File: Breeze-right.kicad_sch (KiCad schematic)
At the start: 103 parts, among them J1 J, SW1 CHOCXHSPCB-1U, SW10 CHOCXHSPCB-1U, SW11 CHOCXHSPCB-1U, SW12 CHOCXHSPCB-1U, SW13 CHOCXHSPCB-1U, SW14 CHOCXHSPCB-1U, SW15 CHOCXHSPCB-1U, SW16 CHOCXHSPCB-1U, SW17 CHOCXHSPCB-1U, SW18 CHOCXHSPCB-1U, SW19 CHOCXHSPCB-1U, SW2 CHOCXHSPCB-1U, SW20 CHOCXHSPCB-1U, SW21 CHOCXHSPCB-1U, SW22 CHOCXHSPCB-1U, SW23 CHOCXHSPCB-1U, SW24 CHOCXHSPCB-1U, SW3 CHOCXHSPCB-1U, SW4 CHOCXHSPCB-1U, SW5 CHOCXHSPCB-1U, SW6 CHOCXHSPCB-1U, SW7 CHOCXHSPCB-1U, SW8 CHOCXHSPCB-1U, SW9 CHOCXHSPCB-1U, U1 NRF Supermini

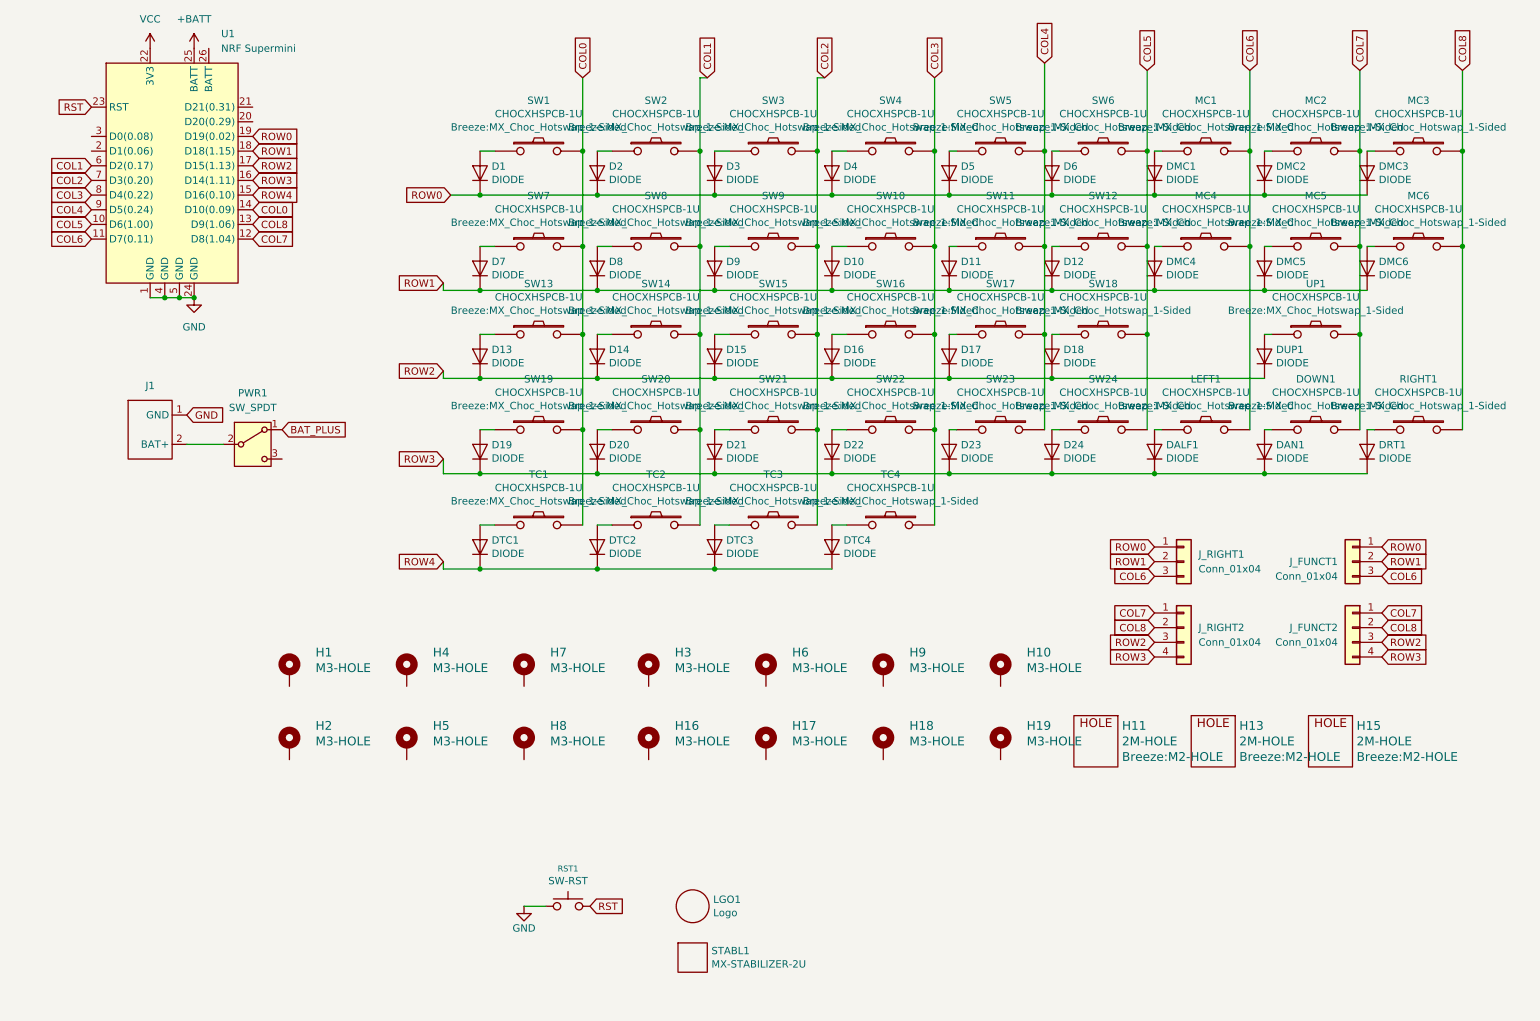
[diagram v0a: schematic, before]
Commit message: done
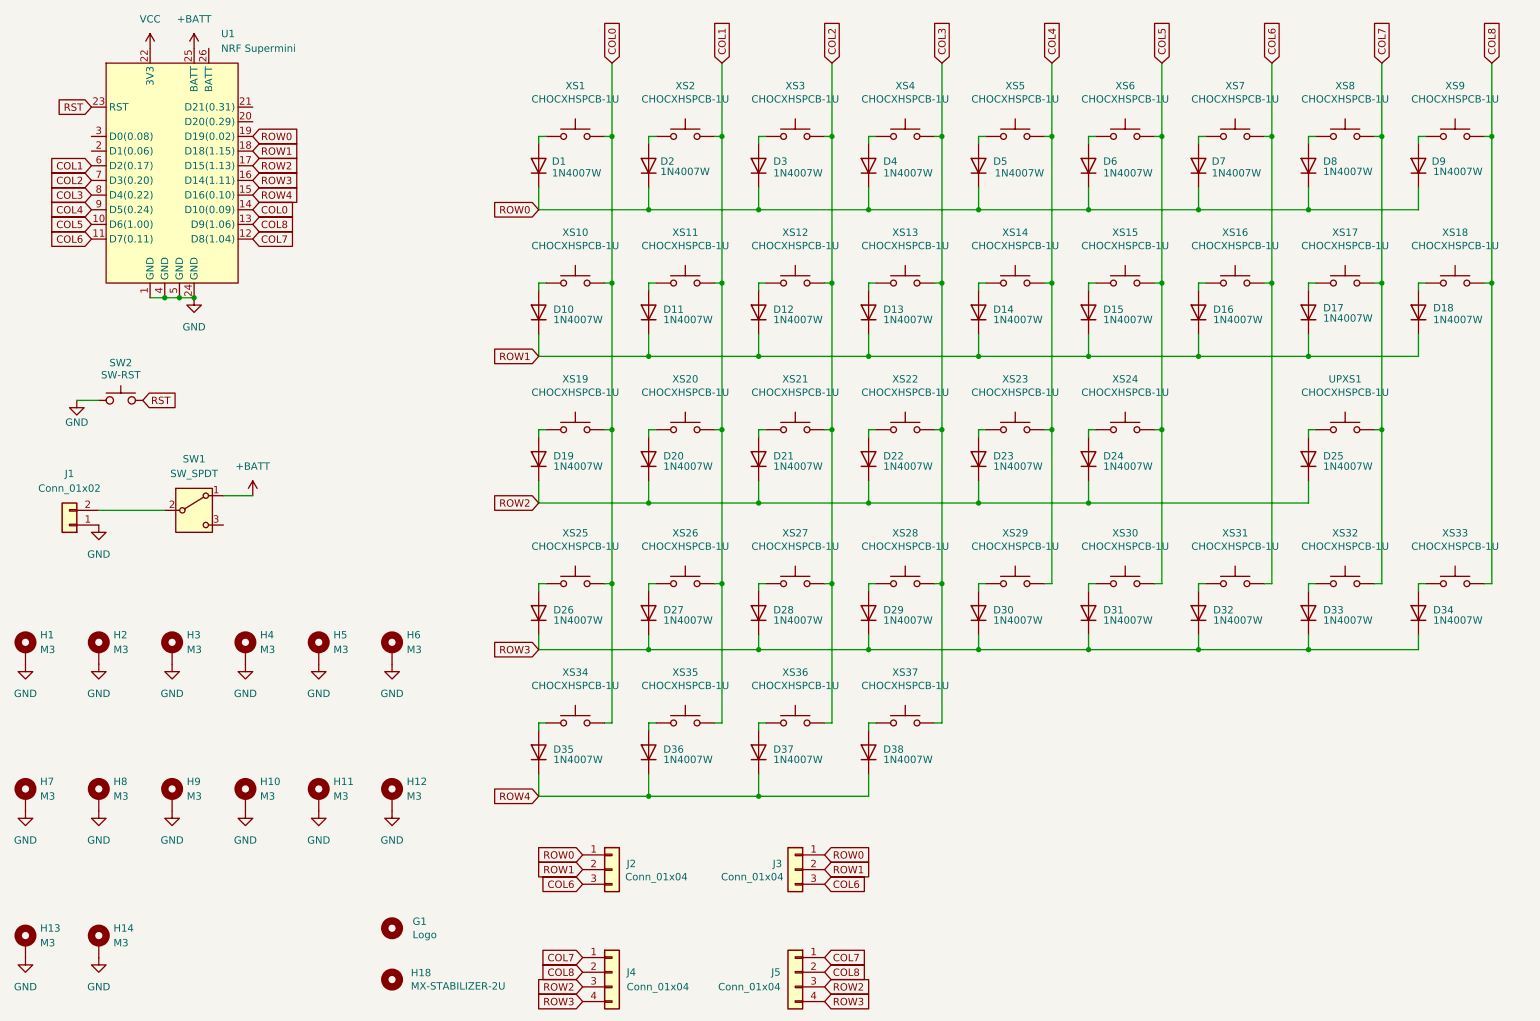
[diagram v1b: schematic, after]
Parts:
- removed H11, H13, H15: 2M-HOLE, Breeze:M2-HOLE, symbol Breeze-rescue:2M-HOLE-Breeze-rescue
- removed H16, H17, H18, H19: M3-HOLE, Breeze:M3-HOLE, symbol Mechanical:MountingHole_Pad
- removed J1: J, Breeze:BATT_PADS, symbol Breeze:BATT_PADS
- removed PWR1: SW_SPDT, Breeze:SS12D00, symbol Switch:SW_SPDT
- added H11, H12, H13, H14: M3, MountingHole:MountingHole_3.2mm_M3_ISO7380_Pad, symbol Mechanical:MountingHole_Pad
- added J1: Conn_01x02, Breeze:BATT_PADS, symbol Connector_Generic:Conn_01x02
- added SW1: SW_SPDT, Breeze:SS12D00, symbol Switch:SW_SPDT
- D1, D2, D3, D4, D5, D6: value DIODE -> 1N4007W; footprint Breeze:SOD-123FL -> Breeze:SOD-123FL_L2.7-W1.8-LS3.7-RD; symbol Breeze-rescue:Diode-cache-Merkaba_Rev0-rescue-Breeze-rescue -> Diode:1N4007
- D10: renamed from D7; value DIODE -> 1N4007W; footprint Breeze:SOD-123FL -> Breeze:SOD-123FL_L2.7-W1.8-LS3.7-RD; symbol Breeze-rescue:Diode-cache-Merkaba_Rev0-rescue-Breeze-rescue -> Diode:1N4007
- D11: renamed from D8; value DIODE -> 1N4007W; footprint Breeze:SOD-123FL -> Breeze:SOD-123FL_L2.7-W1.8-LS3.7-RD; symbol Breeze-rescue:Diode-cache-Merkaba_Rev0-rescue-Breeze-rescue -> Diode:1N4007
- D12: renamed from D9; value DIODE -> 1N4007W; footprint Breeze:SOD-123FL -> Breeze:SOD-123FL_L2.7-W1.8-LS3.7-RD; symbol Breeze-rescue:Diode-cache-Merkaba_Rev0-rescue-Breeze-rescue -> Diode:1N4007
- D13: renamed from D10; value DIODE -> 1N4007W; footprint Breeze:SOD-123FL -> Breeze:SOD-123FL_L2.7-W1.8-LS3.7-RD; symbol Breeze-rescue:Diode-cache-Merkaba_Rev0-rescue-Breeze-rescue -> Diode:1N4007
- D14: renamed from D11; value DIODE -> 1N4007W; footprint Breeze:SOD-123FL -> Breeze:SOD-123FL_L2.7-W1.8-LS3.7-RD; symbol Breeze-rescue:Diode-cache-Merkaba_Rev0-rescue-Breeze-rescue -> Diode:1N4007
- D15: renamed from D12; value DIODE -> 1N4007W; footprint Breeze:SOD-123FL -> Breeze:SOD-123FL_L2.7-W1.8-LS3.7-RD; symbol Breeze-rescue:Diode-cache-Merkaba_Rev0-rescue-Breeze-rescue -> Diode:1N4007
- D16: renamed from DMC4; value DIODE -> 1N4007W; footprint Breeze:SOD-123FL -> Breeze:SOD-123FL_L2.7-W1.8-LS3.7-RD; symbol Breeze-rescue:Diode-cache-Merkaba_Rev0-rescue-Breeze-rescue -> Diode:1N4007
- D17: renamed from DMC5; value DIODE -> 1N4007W; footprint Breeze:SOD-123FL -> Breeze:SOD-123FL_L2.7-W1.8-LS3.7-RD; symbol Breeze-rescue:Diode-cache-Merkaba_Rev0-rescue-Breeze-rescue -> Diode:1N4007
- D18: renamed from DMC6; value DIODE -> 1N4007W; footprint Breeze:SOD-123FL -> Breeze:SOD-123FL_L2.7-W1.8-LS3.7-RD; symbol Breeze-rescue:Diode-cache-Merkaba_Rev0-rescue-Breeze-rescue -> Diode:1N4007
- D19: renamed from D13; value DIODE -> 1N4007W; footprint Breeze:SOD-123FL -> Breeze:SOD-123FL_L2.7-W1.8-LS3.7-RD; symbol Breeze-rescue:Diode-cache-Merkaba_Rev0-rescue-Breeze-rescue -> Diode:1N4007
- D20: renamed from D14; value DIODE -> 1N4007W; footprint Breeze:SOD-123FL -> Breeze:SOD-123FL_L2.7-W1.8-LS3.7-RD; symbol Breeze-rescue:Diode-cache-Merkaba_Rev0-rescue-Breeze-rescue -> Diode:1N4007
- D21: renamed from D15; value DIODE -> 1N4007W; footprint Breeze:SOD-123FL -> Breeze:SOD-123FL_L2.7-W1.8-LS3.7-RD; symbol Breeze-rescue:Diode-cache-Merkaba_Rev0-rescue-Breeze-rescue -> Diode:1N4007
- D22: renamed from D16; value DIODE -> 1N4007W; footprint Breeze:SOD-123FL -> Breeze:SOD-123FL_L2.7-W1.8-LS3.7-RD; symbol Breeze-rescue:Diode-cache-Merkaba_Rev0-rescue-Breeze-rescue -> Diode:1N4007
- D23: renamed from D17; value DIODE -> 1N4007W; footprint Breeze:SOD-123FL -> Breeze:SOD-123FL_L2.7-W1.8-LS3.7-RD; symbol Breeze-rescue:Diode-cache-Merkaba_Rev0-rescue-Breeze-rescue -> Diode:1N4007
- D24: renamed from D18; value DIODE -> 1N4007W; footprint Breeze:SOD-123FL -> Breeze:SOD-123FL_L2.7-W1.8-LS3.7-RD; symbol Breeze-rescue:Diode-cache-Merkaba_Rev0-rescue-Breeze-rescue -> Diode:1N4007
- D25: renamed from DUP1; value DIODE -> 1N4007W; footprint Breeze:SOD-123FL -> Breeze:SOD-123FL_L2.7-W1.8-LS3.7-RD; symbol Breeze-rescue:Diode-cache-Merkaba_Rev0-rescue-Breeze-rescue -> Diode:1N4007
- D26: renamed from D19; value DIODE -> 1N4007W; footprint Breeze:SOD-123FL -> Breeze:SOD-123FL_L2.7-W1.8-LS3.7-RD; symbol Breeze-rescue:Diode-cache-Merkaba_Rev0-rescue-Breeze-rescue -> Diode:1N4007
- D27: renamed from D20; value DIODE -> 1N4007W; footprint Breeze:SOD-123FL -> Breeze:SOD-123FL_L2.7-W1.8-LS3.7-RD; symbol Breeze-rescue:Diode-cache-Merkaba_Rev0-rescue-Breeze-rescue -> Diode:1N4007
- D28: renamed from D21; value DIODE -> 1N4007W; footprint Breeze:SOD-123FL -> Breeze:SOD-123FL_L2.7-W1.8-LS3.7-RD; symbol Breeze-rescue:Diode-cache-Merkaba_Rev0-rescue-Breeze-rescue -> Diode:1N4007
- D29: renamed from D22; value DIODE -> 1N4007W; footprint Breeze:SOD-123FL -> Breeze:SOD-123FL_L2.7-W1.8-LS3.7-RD; symbol Breeze-rescue:Diode-cache-Merkaba_Rev0-rescue-Breeze-rescue -> Diode:1N4007
- D30: renamed from D23; value DIODE -> 1N4007W; footprint Breeze:SOD-123FL -> Breeze:SOD-123FL_L2.7-W1.8-LS3.7-RD; symbol Breeze-rescue:Diode-cache-Merkaba_Rev0-rescue-Breeze-rescue -> Diode:1N4007
- D31: renamed from D24; value DIODE -> 1N4007W; footprint Breeze:SOD-123FL -> Breeze:SOD-123FL_L2.7-W1.8-LS3.7-RD; symbol Breeze-rescue:Diode-cache-Merkaba_Rev0-rescue-Breeze-rescue -> Diode:1N4007
- D32: renamed from DALF1; value DIODE -> 1N4007W; footprint Breeze:SOD-123FL -> Breeze:SOD-123FL_L2.7-W1.8-LS3.7-RD; symbol Breeze-rescue:Diode-cache-Merkaba_Rev0-rescue-Breeze-rescue -> Diode:1N4007
- D33: renamed from DAN1; value DIODE -> 1N4007W; footprint Breeze:SOD-123FL -> Breeze:SOD-123FL_L2.7-W1.8-LS3.7-RD; symbol Breeze-rescue:Diode-cache-Merkaba_Rev0-rescue-Breeze-rescue -> Diode:1N4007
- D34: renamed from DRT1; value DIODE -> 1N4007W; footprint Breeze:SOD-123FL -> Breeze:SOD-123FL_L2.7-W1.8-LS3.7-RD; symbol Breeze-rescue:Diode-cache-Merkaba_Rev0-rescue-Breeze-rescue -> Diode:1N4007
- D35: renamed from DTC1; value DIODE -> 1N4007W; footprint Breeze:SOD-123FL -> Breeze:SOD-123FL_L2.7-W1.8-LS3.7-RD; symbol Breeze-rescue:Diode-cache-Merkaba_Rev0-rescue-Breeze-rescue -> Diode:1N4007
- D36: renamed from DTC2; value DIODE -> 1N4007W; footprint Breeze:SOD-123FL -> Breeze:SOD-123FL_L2.7-W1.8-LS3.7-RD; symbol Breeze-rescue:Diode-cache-Merkaba_Rev0-rescue-Breeze-rescue -> Diode:1N4007
- D37: renamed from DTC3; value DIODE -> 1N4007W; footprint Breeze:SOD-123FL -> Breeze:SOD-123FL_L2.7-W1.8-LS3.7-RD; symbol Breeze-rescue:Diode-cache-Merkaba_Rev0-rescue-Breeze-rescue -> Diode:1N4007
- D38: renamed from DTC4; value DIODE -> 1N4007W; footprint Breeze:SOD-123FL -> Breeze:SOD-123FL_L2.7-W1.8-LS3.7-RD; symbol Breeze-rescue:Diode-cache-Merkaba_Rev0-rescue-Breeze-rescue -> Diode:1N4007
- D7: renamed from DMC1; value DIODE -> 1N4007W; footprint Breeze:SOD-123FL -> Breeze:SOD-123FL_L2.7-W1.8-LS3.7-RD; symbol Breeze-rescue:Diode-cache-Merkaba_Rev0-rescue-Breeze-rescue -> Diode:1N4007
- D8: renamed from DMC2; value DIODE -> 1N4007W; footprint Breeze:SOD-123FL -> Breeze:SOD-123FL_L2.7-W1.8-LS3.7-RD; symbol Breeze-rescue:Diode-cache-Merkaba_Rev0-rescue-Breeze-rescue -> Diode:1N4007
- D9: renamed from DMC3; value DIODE -> 1N4007W; footprint Breeze:SOD-123FL -> Breeze:SOD-123FL_L2.7-W1.8-LS3.7-RD; symbol Breeze-rescue:Diode-cache-Merkaba_Rev0-rescue-Breeze-rescue -> Diode:1N4007
- G1: renamed from LGO1; symbol Breeze-rescue:Logo-Breeze-rescue -> Mechanical:MountingHole; now left out of the parts list
- H1, H10, H3, H4, H6, H7, H9: value M3-HOLE -> M3; footprint Breeze:M3-HOLE -> MountingHole:MountingHole_3.2mm_M3_ISO7380_Pad
- H18: renamed from STABL1; symbol Breeze-rescue:MX-STABILIZER-2U-Merkaba_Rev0-rescue-Breeze-rescue -> Mechanical:MountingHole; now left out of the parts list
- H2, H5, H8: value M3-HOLE -> M3; footprint Breeze:M3-HOLE -> MountingHole:MountingHole_3.2mm_M3_ISO7380_Pad_TopOnly
- UPXS1: renamed from UP1; symbol Breeze-rescue:CHOCXHSPCB-1U-cache-Merkaba_Rev0-rescue-Breeze-rescue -> Switch:SW_Push
- XS1: renamed from SW1; symbol Breeze-rescue:CHOCXHSPCB-1U-cache-Merkaba_Rev0-rescue-Breeze-rescue -> Switch:SW_Push
- XS10: renamed from SW7; symbol Breeze-rescue:CHOCXHSPCB-1U-cache-Merkaba_Rev0-rescue-Breeze-rescue -> Switch:SW_Push
- XS11: renamed from SW8; symbol Breeze-rescue:CHOCXHSPCB-1U-cache-Merkaba_Rev0-rescue-Breeze-rescue -> Switch:SW_Push
- XS12: renamed from SW9; symbol Breeze-rescue:CHOCXHSPCB-1U-cache-Merkaba_Rev0-rescue-Breeze-rescue -> Switch:SW_Push
- XS13: renamed from SW10; symbol Breeze-rescue:CHOCXHSPCB-1U-cache-Merkaba_Rev0-rescue-Breeze-rescue -> Switch:SW_Push
- XS14: renamed from SW11; symbol Breeze-rescue:CHOCXHSPCB-1U-cache-Merkaba_Rev0-rescue-Breeze-rescue -> Switch:SW_Push
- XS15: renamed from SW12; symbol Breeze-rescue:CHOCXHSPCB-1U-cache-Merkaba_Rev0-rescue-Breeze-rescue -> Switch:SW_Push
- XS16: renamed from MC4; symbol Breeze-rescue:CHOCXHSPCB-1U-cache-Merkaba_Rev0-rescue-Breeze-rescue -> Switch:SW_Push
- XS17: renamed from MC5; symbol Breeze-rescue:CHOCXHSPCB-1U-cache-Merkaba_Rev0-rescue-Breeze-rescue -> Switch:SW_Push
- XS18: renamed from MC6; symbol Breeze-rescue:CHOCXHSPCB-1U-cache-Merkaba_Rev0-rescue-Breeze-rescue -> Switch:SW_Push
- XS19: renamed from SW13; symbol Breeze-rescue:CHOCXHSPCB-1U-cache-Merkaba_Rev0-rescue-Breeze-rescue -> Switch:SW_Push
- XS2: renamed from SW2; symbol Breeze-rescue:CHOCXHSPCB-1U-cache-Merkaba_Rev0-rescue-Breeze-rescue -> Switch:SW_Push
- XS20: renamed from SW14; symbol Breeze-rescue:CHOCXHSPCB-1U-cache-Merkaba_Rev0-rescue-Breeze-rescue -> Switch:SW_Push
- XS21: renamed from SW15; symbol Breeze-rescue:CHOCXHSPCB-1U-cache-Merkaba_Rev0-rescue-Breeze-rescue -> Switch:SW_Push
- XS22: renamed from SW16; symbol Breeze-rescue:CHOCXHSPCB-1U-cache-Merkaba_Rev0-rescue-Breeze-rescue -> Switch:SW_Push
- XS23: renamed from SW17; symbol Breeze-rescue:CHOCXHSPCB-1U-cache-Merkaba_Rev0-rescue-Breeze-rescue -> Switch:SW_Push
- XS24: renamed from SW18; symbol Breeze-rescue:CHOCXHSPCB-1U-cache-Merkaba_Rev0-rescue-Breeze-rescue -> Switch:SW_Push
- XS25: renamed from SW19; symbol Breeze-rescue:CHOCXHSPCB-1U-cache-Merkaba_Rev0-rescue-Breeze-rescue -> Switch:SW_Push
- XS26: renamed from SW20; symbol Breeze-rescue:CHOCXHSPCB-1U-cache-Merkaba_Rev0-rescue-Breeze-rescue -> Switch:SW_Push
- XS27: renamed from SW21; symbol Breeze-rescue:CHOCXHSPCB-1U-cache-Merkaba_Rev0-rescue-Breeze-rescue -> Switch:SW_Push
- XS28: renamed from SW22; symbol Breeze-rescue:CHOCXHSPCB-1U-cache-Merkaba_Rev0-rescue-Breeze-rescue -> Switch:SW_Push
- XS29: renamed from SW23; symbol Breeze-rescue:CHOCXHSPCB-1U-cache-Merkaba_Rev0-rescue-Breeze-rescue -> Switch:SW_Push
- XS3: renamed from SW3; symbol Breeze-rescue:CHOCXHSPCB-1U-cache-Merkaba_Rev0-rescue-Breeze-rescue -> Switch:SW_Push
- XS30: renamed from SW24; symbol Breeze-rescue:CHOCXHSPCB-1U-cache-Merkaba_Rev0-rescue-Breeze-rescue -> Switch:SW_Push
- XS31: renamed from LEFT1; symbol Breeze-rescue:CHOCXHSPCB-1U-cache-Merkaba_Rev0-rescue-Breeze-rescue -> Switch:SW_Push
- XS32: renamed from DOWN1; symbol Breeze-rescue:CHOCXHSPCB-1U-cache-Merkaba_Rev0-rescue-Breeze-rescue -> Switch:SW_Push
- XS33: renamed from RIGHT1; symbol Breeze-rescue:CHOCXHSPCB-1U-cache-Merkaba_Rev0-rescue-Breeze-rescue -> Switch:SW_Push
- XS34: renamed from TC1; symbol Breeze-rescue:CHOCXHSPCB-1U-cache-Merkaba_Rev0-rescue-Breeze-rescue -> Switch:SW_Push
- XS35: renamed from TC2; symbol Breeze-rescue:CHOCXHSPCB-1U-cache-Merkaba_Rev0-rescue-Breeze-rescue -> Switch:SW_Push
- XS36: renamed from TC3; symbol Breeze-rescue:CHOCXHSPCB-1U-cache-Merkaba_Rev0-rescue-Breeze-rescue -> Switch:SW_Push
- XS37: renamed from TC4; symbol Breeze-rescue:CHOCXHSPCB-1U-cache-Merkaba_Rev0-rescue-Breeze-rescue -> Switch:SW_Push
- XS4: renamed from SW4; symbol Breeze-rescue:CHOCXHSPCB-1U-cache-Merkaba_Rev0-rescue-Breeze-rescue -> Switch:SW_Push
- XS5: renamed from SW5; symbol Breeze-rescue:CHOCXHSPCB-1U-cache-Merkaba_Rev0-rescue-Breeze-rescue -> Switch:SW_Push
- XS6: renamed from SW6; symbol Breeze-rescue:CHOCXHSPCB-1U-cache-Merkaba_Rev0-rescue-Breeze-rescue -> Switch:SW_Push
- XS7: renamed from MC1; symbol Breeze-rescue:CHOCXHSPCB-1U-cache-Merkaba_Rev0-rescue-Breeze-rescue -> Switch:SW_Push
- XS8: renamed from MC2; symbol Breeze-rescue:CHOCXHSPCB-1U-cache-Merkaba_Rev0-rescue-Breeze-rescue -> Switch:SW_Push
- XS9: renamed from MC3; symbol Breeze-rescue:CHOCXHSPCB-1U-cache-Merkaba_Rev0-rescue-Breeze-rescue -> Switch:SW_Push
- renumbered J_RIGHT1 to J2, J_FUNCT1 to J3, J_RIGHT2 to J4, J_FUNCT2 to J5, RST1 to SW2
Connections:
- net +BATT: now also SW1.1 (A)
- net GND: now also H1.1, H10.1, H2.1, H3.1, H4.1, H5.1, H6.1, H7.1, H8.1, H9.1, H11.1, H12.1, H13.1, H14.1, J1.1 (Pin_1)
- new net: J1.2 (Pin_2), SW1.2 (B)
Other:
- moved on the sheet: D1, D10, D11, D12, D13, D14, D15, D16, D17, D18, D19, D2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
